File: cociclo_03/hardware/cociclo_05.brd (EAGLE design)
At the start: 42.2 x 43.9 mm, 15 parts

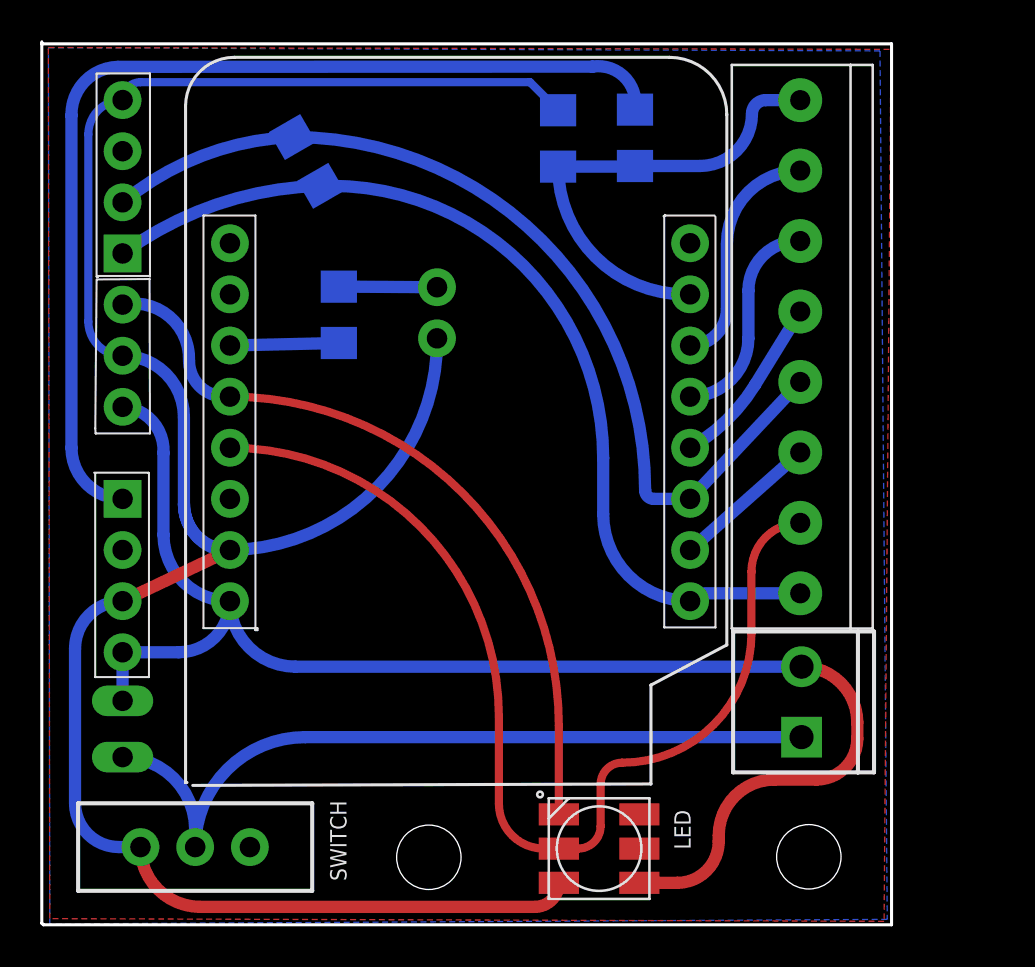
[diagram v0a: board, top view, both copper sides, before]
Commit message: début de la version 05 et fichiers grb
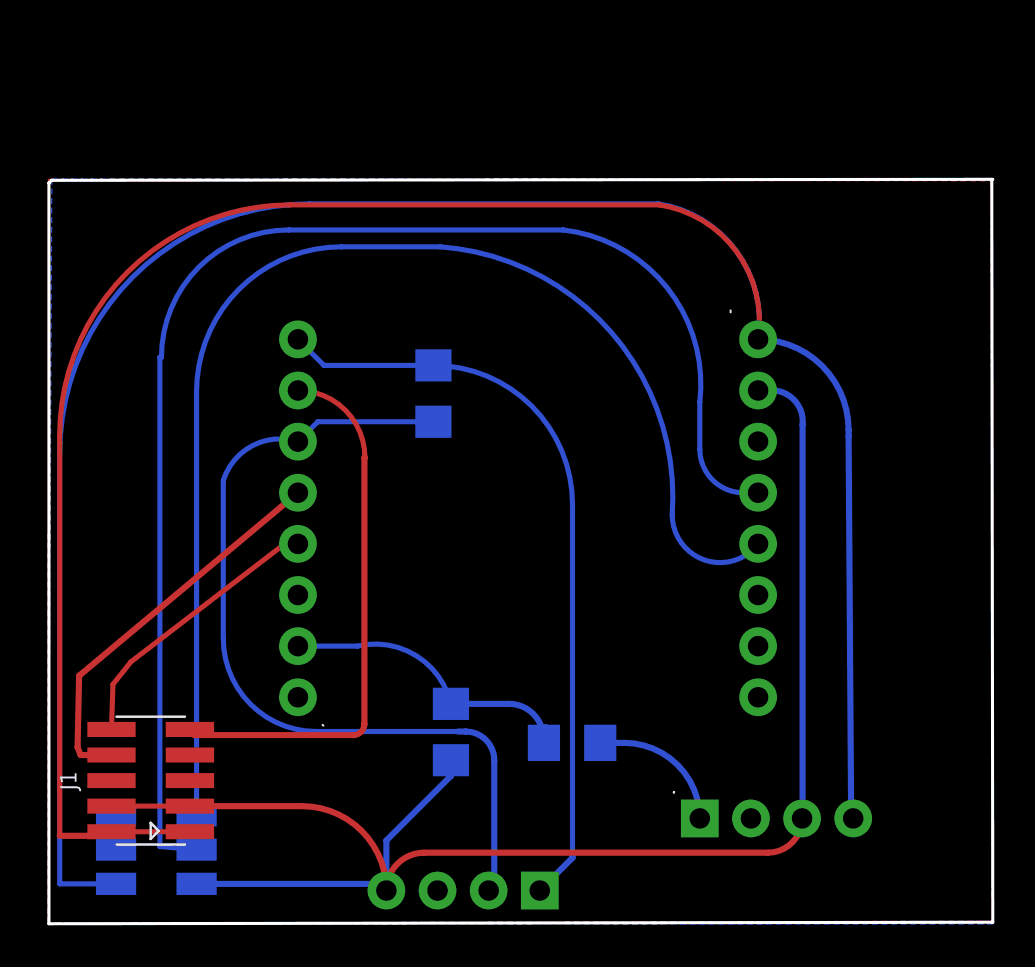
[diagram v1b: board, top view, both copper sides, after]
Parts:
- removed DEL: (no value), SparkFun-Connectors:1X03
- removed JP3: (no value), adafruit:1X08-3.5MM
- removed JP6: (no value), SparkFun-Connectors:SCREWTERMINAL-3.5MM-2
- removed JSPEAKER: (no value), SparkFun-Connectors:1X02
- removed PWR: (no value), SparkFun-Connectors:1X02_LOCK_LONGPADS
- removed R3: 100 ohms, SparkFun-Resistors:1206
- removed SWITCH: (no value), SparkFun-Electromechanical:SWITCH-SPDT_KIT
- added J1: PMS7003, Board-to-Board (rev18a):621X1021021
- moved DHT11 37.8 mm to (24.5, 1.70), turned to 0 degrees
- moved MQ-7 32.8 mm to (32.4, 5.28), turned to 180 degrees
- moved R2 30.2 mm to (26.1, 9.04), turned to 0 degrees
- moved R1 30.0 mm to (20.1, 9.58), turned to 90 degrees
- moved JP1 29.8 mm to (12.5, 11.3), turned to 90 degrees
- moved JP2 29.3 mm to (35.3, 29.1), turned to 270 degrees
- moved LED 22.0 mm to (5.44, 3.73), flipped to the bottom
- moved R6 13.1 mm to (19.2, 26.4), turned to 270 degrees
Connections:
- removed net GPIO12: JP2.6, R3.1
- removed net N$11: JP1.5, JP3.5
- removed net N$12: JP1.4, JP3.6
- removed net N$13: JP1.3, JP3.7
- removed net N$4: JSPEAKER.1, R3.2
- removed net N$8: JP1.7, JP3.3
- removed net N$9: JP6.1, PWR.2, SWITCH.2
- new net 10SET: J1.9, JP1.7
- new net 7RX: J1.8, JP1.5
- new net 9TX: J1.10, JP1.4
- net +5V: now also J1.1, J1.2; no longer DEL.3, JP6.2, PWR.1
- net ADC: no longer JP3.8
- net CH_PD: no longer JP3.1
- net D2: no longer DEL.1
- net GND: now also J1.3, J1.4; no longer DEL.2, JSPEAKER.2, SWITCH.3
- net GPIO14: no longer JP3.4
- net N$10: no longer JP3.2
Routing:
- net +5V: track 69.0 -> 162.6 mm
- net MQ7ANALOG: track 50.1 -> 6.50 mm
- net N$9: track 38.4 -> 0.00 mm
- net GND: track 110.4 -> 78.0 mm
- net 10SET: track 0.00 -> 27.0 mm
- net D2: track 34.6 -> 58.2 mm
- net 7RX: track 0.00 -> 19.8 mm
- net N$10: track 48.8 -> 65.8 mm
- net 9TX: track 0.00 -> 14.0 mm
- net N$13: track 11.0 -> 0.00 mm
- net N$12: track 10.1 -> 0.00 mm
- net N$11: track 8.77 -> 0.00 mm
- net ADC: track 23.6 -> 15.1 mm
- net N$8: track 7.31 -> 0.00 mm
- net CH_PD: track 44.6 -> 37.4 mm
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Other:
- board size 42.2 x 43.9 mm -> 46.9 x 37 mm
- board text added: "/Users/uqam/Desktop/logo_unloquerVector_s.bmp"
- board text added: "v0.5"
- board text removed: "0.1k"
- board text removed: "5V"
- board text removed: "SPK"
- board text removed: "v0.3"
